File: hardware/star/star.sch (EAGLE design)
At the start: 520 parts, among them IC1 MAX481CSA, IC10 MAX481CSA, IC11 MAX481CSA, IC12 MAX481CSA, IC13 MAX481CSA, IC14 MAX481CSA, IC15 MAX481CSA, IC16 MAX481CSA, IC17 MAX481CSA, IC18 MAX481CSA, IC19 MAX481CSA, IC2 LD117AS12TR, IC20 MAX481CSA, IC21 MAX481CSA, IC22 LD117AS12TR, IC23 LD117AS12TR, IC3 MAX481CSA, IC4 MAX481CSA, IC5 MAX481CSA, IC6 MAX481CSA, IC7 MAX481CSA, IC8 MAX481CSA, IC9 MAX481CSA

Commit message: Progress
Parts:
- removed ACCESSORY, ACCESSORY_GPIO: (no value), pinhead:PINHD-1X5
- removed C100, C101, C102, C103, C104, C105, C106, C107, C108, C109, C110, C111, C112, C113, C114, C115, C116, C117, C118, C119, C120, C121, C122, C123, C124, C37, C38, C39, C40, C41, C42, C43, C44, C45, C46, C47, C48, C49, C50, C51, C52, C53, C54, C55, C56, C57, C58, C59, C60, C61, C62, C63, C64, C65, C66, C67, C68, C73, C74, C75, C76, C77, C78, C79, C80, C81, C82, C83, C84, C85, C86, C87, C88, C93, C94, C95, C96, C97, C98, C99: 1nf, rcl:C-USC0603
- removed C24, C25, C26, C27, C28, C29, C30, C31, C32, C33, C90: 1uf, rcl:C-USC0805
- removed C34, C91, C92: 10uf, rcl:C-USC0603
- removed C69, C70, C71, C72: 2200uf, rcl:CPOL-USE5-13
- removed D10, D11, D12, D13, D14, D15, D16, D17, D18, D19, D20, D21, D22, D23, D24, D25, D26, D27, D28, D29, D30, D31, D32, D33, D34, D35, D36, D37, D38, D39, D40, D41, D42, D43, D44, D45, D46, D47, D48, D49, D50, D51, D52, D53, D54, D55, D56, D57, D58, D59, D60, D61, D62, D63, D64, D65, D66, D67, D68, D69, D70, D71, D72, D73, D74, D75, D76, D77, D78, D79, D80: (no value), SparkFun-LED:LED0603
- removed D81, D86: red, SparkFun-LED:LED0603
- removed D82, D87: green, SparkFun-LED:LED0603
- removed D83, D88: blue, SparkFun-LED:LED0603
- removed D84, D89: white, SparkFun-LED:LED0603
- removed D85, D90: yellow, SparkFun-LED:LED0603
- removed GAME_INTERFACE: B12B-PH-K, con-jst-ph:B12B-PH-K
- removed IC10, IC11, IC12, IC13, IC14, IC15, IC16, IC17, IC18, IC19, IC20, IC21, IC5, IC6, IC7, IC8, IC9: MAX481CSA, maxim:MAX481CSA
- removed IC23: LD117AS12TR, v-reg:LD117AS12TR
- removed J1: (no value), SparkFun-Connectors:CONN_02JST-PTH-2
- removed JP1: (no value), pinhead:PINHD-1X2
- removed JP2: (no value), pinhead:PINHD-1X4
- removed NEBULA_B, NEBULA_C, NEBULA_D, NEBULA_E, NEBULA_F, NEBULA_G, NEBULA_H: MCP23017-E/SO, MCP23017-E_SO:MCP23017-E/SO
- removed R100, R101, R102, R133, R134, R135, R136, R137, R50, R51, R52, R53, R66, R67, R69, R70, R71, R72, R73, R74, R75, R76, R77, R78, R79, R80, R81, R82, R87, R88, R89, R90, R91, R92, R93, R94, R95, R96, R97, R98, R99: 10k, rcl:R-US_R0603
- removed R103, R104, R105, R106, R140, R141, R142, R143, R144, R145, R146, R147, R148, R149, R150, R151, R152, R153, R154, R155, R156, R157, R158, R159, R160, R161, R162, R163, R164, R165, R166, R167, R168, R169, R170, R171, R172, R173, R174, R175, R176, R177, R178, R179, R180, R181, R182, R183, R184, R185, R186, R187, R188, R189, R190, R191, R192, R193, R194, R195, R196, R197, R198, R199, R200, R201, R202, R203, R204, R205, R206, R207, R208, R209, R210, R211, R212, R213, R214, R215, R216, R217, R218, R219, R54, R55, R56, R57, R58, R59, R60, R61, R62, R63, R64, R65, R83, R84, R85, R86: 68, rcl:R-US_R0603
- removed R107, R108, R109, R110, R111, R112, R113, R114, R115, R116, R117, R118, R119, R120, R121, R122, R123, R124: 120, rcl:R-US_R0603
- removed R125, R126, R127, R128, R129: 1k, rcl:R-US_R0603
- removed R138, R68: 10, rcl:R-US_R1206
- removed S1, S2, S3, S4, S5: MOMENTARY-SWITCH-SPST-PTH-6.0MM, SparkFun-Switches:MOMENTARY-SWITCH-SPST-PTH-6.0MM
- removed STAR_10, STAR_11, STAR_12, STAR_13, STAR_14, STAR_15, STAR_16, STAR_17, STAR_18, STAR_19, STAR_2, STAR_20, STAR_3, STAR_4, STAR_5, STAR_6, STAR_7, STAR_8, STAR_9: B8B-PH-K, con-jst-ph:B8B-PH-K
- removed ULN10, ULN11, ULN12, ULN2, ULN3, ULN4, ULN5, ULN6, ULN7, ULN8, ULN9: (no value), SparkFun-IC-Special-Function:ULN2803SOICW
- added K1, K2: T90-12VDC-TL-A, relay:JT1A-PCB-DC12V
- added T1, T2, T3, T4: T_PNP_MMBT5401_CHANGJ_SOT23-BEC, JLC PCB Basic Parts_loc:T_PNP_MMBT5401_CHANGJ_SOT23-BEC
- added U1: TCLT1600, TCLT1600:TCLT1600
- added ULN1: (no value), SparkFun-IC-Special-Function:ULN2803SOICW
- added X1: MKDSN1,5/2-5,08, con-phoenix-508:MKDSN1,5/2-5,08
- added X3: MKDSN1,5/5-5,08, con-phoenix-508:MKDSN1,5/5-5,08
- C10, C11, C12, C9: value 10uf -> C_100UF/6.3V_1206; device rcl:C-USC0603 -> JLC PCB Basic Parts_loc:C_100UF/6.3V_1206; LCSC_PART C19702 -> (none)
- C13: value 10uf -> C_1NF/2KV_1206; device rcl:C-USC0603 -> JLC PCB Basic Parts_loc:C_1NF/2KV_1206; LCSC_PART C19702 -> (none)
- C15, C19, C21, C23: value 1uf -> C_100PF/50V_0603; device rcl:C-USC0805 -> JLC PCB Basic Parts_loc:C_100PF/50V_0603; LCSC_PART C15849 -> (none)
- C16, C17: value 1uf -> C_1NF/50V_0603; device rcl:C-USC0805 -> JLC PCB Basic Parts_loc:C_1NF/50V_0603; LCSC_PART C15849 -> (none)
- C18, C20, C22: value 1uf -> C_1NF/2KV_1206; device rcl:C-USC0805 -> JLC PCB Basic Parts_loc:C_1NF/2KV_1206; LCSC_PART C15849 -> (none)
- C7: value 10uf -> C_1NF/50V_0603; device rcl:C-USC0603 -> JLC PCB Basic Parts_loc:C_1NF/50V_0603; LCSC_PART C19702 -> (none)
- D1: value (none) -> red; JLC_ROTATION (none) -> 180
- D6: value (none) -> green; JLC_ROTATION (none) -> 180; LCSC_PART C2286 -> C72043
- D7: value (none) -> green; JLC_ROTATION (none) -> 180
- D8: value (none) -> green; JLC_ROTATION (none) -> 180; LCSC_PART C72041 -> C72043
- D9: value (none) -> green; JLC_ROTATION (none) -> 180; LCSC_PART C2290 -> C72043
- D91, D92, D93, D94: JLC_ROTATION (none) -> 180
- IC3: value MAX481CSA -> 74HCT08D; device maxim:MAX481CSA -> 74xx-eu:74HCT08D; LCSC_PART C8963 -> C5593
- IC4: value MAX481CSA -> 7404D; device maxim:MAX481CSA -> 74xx-us:7404D; LCSC_PART C8963 -> C5590
- R10, R11, R12, R13: value 10k -> R_4.7K_1206; device rcl:R-US_R0603 -> JLC PCB Basic Parts_loc:R_4.7K_1206; LCSC_PART C25804 -> (none)
- R14, R21, R23, R30, R32, R37, R39, R44: value 10k -> R_2K_0603; device rcl:R-US_R0603 -> JLC PCB Basic Parts_loc:R_2K_0603; LCSC_PART C25804 -> (none)
- R15, R24, R33, R40: value 10k -> R_10R_0603; device rcl:R-US_R0603 -> JLC PCB Basic Parts_loc:R_10R_0603; LCSC_PART C25804 -> (none)
- R16, R25, R34, R41: value 10k -> R_12K_0603; device rcl:R-US_R0603 -> JLC PCB Basic Parts_loc:R_12K_0603; LCSC_PART C25804 -> (none)
- R17, R28, R35, R42: value 10k -> R_2.7K_0603; device rcl:R-US_R0603 -> JLC PCB Basic Parts_loc:R_2.7K_0603; LCSC_PART C25804 -> (none)
- R18, R29, R36, R43: value 10k -> R_1K_0603; device rcl:R-US_R0603 -> JLC PCB Basic Parts_loc:R_1K_0603; LCSC_PART C25804 -> (none)
- R19, R20: value 10k -> R_5.1K_0603; device rcl:R-US_R0603 -> JLC PCB Basic Parts_loc:R_5.1K_0603; LCSC_PART C25804 -> (none)
- R2: value 120 -> R_150R_0603; device rcl:R-US_R0603 -> JLC PCB Basic Parts_loc:R_150R_0603; LCSC_PART C22787 -> (none)
- R22, R31, R38, R9: value 10k -> R_7.5K_0603; device rcl:R-US_R0603 -> JLC PCB Basic Parts_loc:R_7.5K_0603; LCSC_PART C25804 -> (none)
- R45, R46, R47, R48: value 10k -> R_6.2K_0603; device rcl:R-US_R0603 -> JLC PCB Basic Parts_loc:R_6.2K_0603; LCSC_PART C25804 -> (none)
- R49: value 10k -> R_0R_0603; device rcl:R-US_R0603 -> JLC PCB Basic Parts_loc:R_0R_0603; LCSC_PART C25804 -> (none)
- R7, R8: value 10k -> 1k; LCSC_PART C25804 -> C21190
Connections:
- removed net B0: NEBULA_B.GPA0, ULN5.8
- removed net B1: NEBULA_B.GPA1, ULN5.7
- removed net B10: NEBULA_B.GPB2, ULN6.6
- removed net B11: NEBULA_B.GPB3, ULN6.5
- removed net B12: NEBULA_B.GPB4, ULN6.4
- removed net B13: NEBULA_B.GPB5, ULN6.3
- removed net B14: NEBULA_B.GPB6, ULN6.2
- removed net B15: NEBULA_B.GPB7, ULN6.1
- removed net B2: NEBULA_B.GPA2, ULN5.6
- removed net B3: NEBULA_B.GPA3, ULN5.5
- removed net B4: NEBULA_B.GPA4, ULN5.4
- removed net B5: NEBULA_B.GPA5, ULN5.3
- removed net B6: NEBULA_B.GPA6, ULN5.2
- removed net B7: NEBULA_B.GPA7, ULN5.1
- removed net B8: NEBULA_B.GPB0, ULN6.8
- removed net B9: NEBULA_B.GPB1, ULN6.7
- removed net C0: NEBULA_C.GPA0, ULN7.8
- removed net C1: NEBULA_C.GPA1, ULN7.7
- removed net C10: NEBULA_C.GPB2, ULN8.6
- removed net C11: NEBULA_C.GPB3, ULN8.5
- removed net C12: NEBULA_C.GPB4, ULN8.4
- removed net C13: NEBULA_C.GPB5, ULN8.3
- removed net C14: NEBULA_C.GPB6, ULN8.2
- removed net C15: NEBULA_C.GPB7, ULN8.1
- removed net C2: NEBULA_C.GPA2, ULN7.6
- removed net C3: NEBULA_C.GPA3, ULN7.5
- removed net C4: NEBULA_C.GPA4, ULN7.4
- removed net C5: NEBULA_C.GPA5, ULN7.3
- removed net C6: NEBULA_C.GPA6, ULN7.2
- removed net C7: NEBULA_C.GPA7, ULN7.1
- removed net C8: NEBULA_C.GPB0, ULN8.8
- removed net C9: NEBULA_C.GPB1, ULN8.7
- removed net D0: NEBULA_D.GPA0, ULN9.8
- removed net D1: NEBULA_D.GPA1, ULN9.7
- removed net D10: NEBULA_D.GPB2, ULN10.6
- removed net D11: NEBULA_D.GPB3, ULN10.5
- removed net D12: NEBULA_D.GPB4, ULN10.4
- removed net D13: NEBULA_D.GPB5, ULN10.3
- removed net D14: NEBULA_D.GPB6, ULN10.2
- removed net D15: NEBULA_D.GPB7, ULN10.1
- removed net D2: NEBULA_D.GPA2, ULN9.6
- removed net D3: NEBULA_D.GPA3, ULN9.5
- removed net D4: NEBULA_D.GPA4, ULN9.4
- removed net D5: NEBULA_D.GPA5, ULN9.3
- removed net D6: NEBULA_D.GPA6, ULN9.2
- removed net D7: NEBULA_D.GPA7, ULN9.1
- removed net D8: NEBULA_D.GPB0, ULN10.8
- removed net D9: NEBULA_D.GPB1, ULN10.7
- removed net E0: NEBULA_E.GPA0, ULN11.8
- removed net E1: NEBULA_E.GPA1, ULN11.7
- removed net E10: NEBULA_E.GPB2, ULN12.6
- removed net E11: NEBULA_E.GPB3, ULN12.5
- removed net E12: NEBULA_E.GPB4, ULN12.4
- removed net E13: NEBULA_E.GPB5, ULN12.3
- removed net E14: NEBULA_E.GPB6, ULN12.2
- removed net E15: NEBULA_E.GPB7, ULN12.1
- removed net E2: NEBULA_E.GPA2, ULN11.6
- removed net E3: NEBULA_E.GPA3, ULN11.5
- removed net E4: NEBULA_E.GPA4, ULN11.4
- removed net E5: NEBULA_E.GPA5, ULN11.3
- removed net E6: NEBULA_E.GPA6, ULN11.2
- removed net E7: NEBULA_E.GPA7, ULN11.1
- removed net E8: NEBULA_E.GPB0, ULN12.8
- removed net E9: NEBULA_E.GPB1, ULN12.7
- removed net F0: IC1G$1.RE/, NEBULA_F.GPA0
- removed net F1: IC1G$1.DE, NEBULA_F.GPA1
- removed net F10: IC7G$1.RE/, NEBULA_F.GPB2
- removed net F11: IC7G$1.DE, NEBULA_F.GPB3
- removed net F12: IC8G$1.RE/, NEBULA_F.GPB4
- removed net F13: IC8G$1.DE, NEBULA_F.GPB5
- removed net F14: IC9G$1.RE/, NEBULA_F.GPB6
- removed net F15: IC9G$1.DE, NEBULA_F.GPB7
- removed net F2: IC3G$1.RE/, NEBULA_F.GPA2
- removed net F3: IC3G$1.DE, NEBULA_F.GPA3
- removed net F4: IC4G$1.RE/, NEBULA_F.GPA4
- removed net F5: IC4G$1.DE, NEBULA_F.GPA5
- removed net F6: IC5G$1.RE/, NEBULA_F.GPA6
- removed net F7: IC5G$1.DE, NEBULA_F.GPA7
- removed net F8: IC6G$1.RE/, NEBULA_F.GPB0
- removed net F9: IC6G$1.DE, NEBULA_F.GPB1
- removed net G0: IC10G$1.RE/, NEBULA_G.GPA0
- removed net G1: IC10G$1.DE, NEBULA_G.GPA1
- removed net G10: IC15G$1.RE/, NEBULA_G.GPB2
- removed net G11: IC15G$1.DE, NEBULA_G.GPB3
- removed net G12: IC16G$1.RE/, NEBULA_G.GPB4
- removed net G13: IC16G$1.DE, NEBULA_G.GPB5
- removed net G14: IC17G$1.RE/, NEBULA_G.GPB6
- removed net G15: IC17G$1.DE, NEBULA_G.GPB7
- removed net G2: IC11G$1.RE/, NEBULA_G.GPA2
- removed net G3: IC11G$1.DE, NEBULA_G.GPA3
- removed net G4: IC12G$1.RE/, NEBULA_G.GPA4
- removed net G5: IC12G$1.DE, NEBULA_G.GPA5
- removed net G6: IC13G$1.RE/, NEBULA_G.GPA6
- removed net G7: IC13G$1.DE, NEBULA_G.GPA7
- removed net G8: IC14G$1.RE/, NEBULA_G.GPB0
- removed net G9: IC14G$1.DE, NEBULA_G.GPB1
- removed net H0: IC18G$1.RE/, NEBULA_H.GPA0
- removed net H1: IC18G$1.DE, NEBULA_H.GPA1
- removed net H10: D88.C, GAME_INTERFACE.4, NEBULA_H.GPB2, R135.2, S3.1
- removed net H11: D90.C, GAME_INTERFACE.5, NEBULA_H.GPB3, R134.2, S4.1
- removed net H12: D89.C, GAME_INTERFACE.6, NEBULA_H.GPB4, R133.2, S5.1
- removed net H13: ACCESSORY_GPIO.2, NEBULA_H.GPB5, ULN2.3
- removed net H14: ACCESSORY_GPIO.3, NEBULA_H.GPB6, ULN2.2
- removed net H15: ACCESSORY_GPIO.4, NEBULA_H.GPB7, ULN2.1
- removed net H2: IC19G$1.RE/, NEBULA_H.GPA2
- removed net H3: IC19G$1.DE, NEBULA_H.GPA3
- removed net H4: IC20G$1.RE/, NEBULA_H.GPA4
- removed net H5: IC20G$1.DE, NEBULA_H.GPA5
- removed net H6: IC21G$1.RE/, NEBULA_H.GPA6
- removed net H7: IC21G$1.DE, NEBULA_H.GPA7
- removed net H8: D86.C, GAME_INTERFACE.2, NEBULA_H.GPB0, R137.2, S1.1
- removed net H9: D87.C, GAME_INTERFACE.3, NEBULA_H.GPB1, R136.2, S2.1
- removed net N$100: D77.C, R99.2
- removed net N$101: D78.C, R100.2
- removed net N$102: D79.C, R101.2
- removed net N$103: D80.C, R102.2
- removed net N$104: R104.2, STAR_18.6
- removed net N$105: R105.2, STAR_19.6
- removed net N$106: R106.2, STAR_20.6
- removed net N$107: R103.2, STAR_17.6
- removed net N$110: IC3G$1.B, R2.2, STAR_2.7
- removed net N$111: IC3G$1.A, R2.1, STAR_2.8
- removed net N$112: IC4G$1.B, R107.2, STAR_3.7
- removed net N$113: IC4G$1.A, R107.1, STAR_3.8
- removed net N$114: IC5G$1.B, R108.2, STAR_4.7
- removed net N$115: IC5G$1.A, R108.1, STAR_4.8
- removed net N$116: IC6G$1.B, R109.2, STAR_5.7
- removed net N$117: IC6G$1.A, R109.1, STAR_5.8
- removed net N$118: IC7G$1.B, R110.2, STAR_6.7
- removed net N$119: IC7G$1.A, R110.1, STAR_6.8
- removed net N$120: IC8G$1.B, R111.2, STAR_7.7
- removed net N$121: IC8G$1.A, R111.1, STAR_7.8
- removed net N$122: IC9G$1.B, R112.2, STAR_8.7
- removed net N$123: IC9G$1.A, R112.1, STAR_8.8
- removed net N$124: IC10G$1.B, R113.2, STAR_9.7
- removed net N$125: IC10G$1.A, R113.1, STAR_9.8
- removed net N$126: IC11G$1.B, R114.2, STAR_10.7
- removed net N$127: IC11G$1.A, R114.1, STAR_10.8
- removed net N$128: IC12G$1.B, R115.2, STAR_11.7
- removed net N$129: IC12G$1.A, R115.1, STAR_11.8
- removed net N$130: IC13G$1.B, R116.2, STAR_12.7
- removed net N$131: IC13G$1.A, R116.1, STAR_12.8
- removed net N$132: IC14G$1.B, R117.2, STAR_13.7
- removed net N$133: IC14G$1.A, R117.1, STAR_13.8
- removed net N$134: IC15G$1.B, R118.2, STAR_14.7
- removed net N$135: IC15G$1.A, R118.1, STAR_14.8
- removed net N$136: IC16G$1.B, R119.2, STAR_15.7
- removed net N$137: IC16G$1.A, R119.1, STAR_15.8
- removed net N$138: IC17G$1.B, R120.2, STAR_16.7
- removed net N$139: IC17G$1.A, R120.1, STAR_16.8
- removed net N$140: IC18G$1.B, R121.2, STAR_17.7
- removed net N$141: IC18G$1.A, R121.1, STAR_17.8
- removed net N$142: IC19G$1.B, R122.2, STAR_18.7
- removed net N$143: IC19G$1.A, R122.1, STAR_18.8
- removed net N$144: IC20G$1.B, R123.2, STAR_19.7
- removed net N$145: IC20G$1.A, R123.1, STAR_19.8
- removed net N$146: IC21G$1.B, R124.2, STAR_20.7
- removed net N$147: IC21G$1.A, R124.1, STAR_20.8
- removed net N$148: ACCESSORY.2, ULN2.16
- removed net N$149: ACCESSORY.3, ULN2.17
- removed net N$150: ACCESSORY.4, ULN2.18
- removed net N$151: D84.A, R129.2
- removed net N$152: D85.A, R128.2
- removed net N$153: D83.A, R127.2
- removed net N$154: D82.A, R126.2
- removed net N$155: D81.A, R125.2
- removed net N$160: C37.1, R143.1, R3.1, ULN3.11
- removed net N$161: C38.1, R142.1, R4.1, ULN3.12
- removed net N$162: C39.1, R141.1, R5.1, ULN3.13
- removed net N$163: C40.1, R140.1, R6.1, ULN3.14
- removed net N$164: C44.1, R10.1, R144.1, ULN3.18
- removed net N$165: C43.1, R145.1, R9.1, ULN3.17
- removed net N$166: C42.1, R146.1, R8.1, ULN3.16
- removed net N$167: C41.1, R147.1, R7.1, ULN3.15
- removed net N$168: R143.2, STAR_1.2
- removed net N$169: R142.2, STAR_1.3
- removed net N$170: R141.2, STAR_1.4
- removed net N$171: R140.2, STAR_1.5
- removed net N$172: R147.2, STAR_2.2
- removed net N$173: R146.2, STAR_2.3
- removed net N$174: R145.2, STAR_2.4
- removed net N$175: R144.2, STAR_2.5
- removed net N$176: R151.2, STAR_3.2
- removed net N$177: R150.2, STAR_3.3
- removed net N$178: R149.2, STAR_3.4
- removed net N$179: R148.2, STAR_3.5
- removed net N$180: R155.2, STAR_4.2
- removed net N$181: R154.2, STAR_4.3
- removed net N$182: R153.2, STAR_4.4
- removed net N$183: R152.2, STAR_4.5
- removed net N$184: C45.1, R11.1, R151.1, ULN4.11
- removed net N$185: C46.1, R12.1, R150.1, ULN4.12
- removed net N$186: C47.1, R13.1, R149.1, ULN4.13
- removed net N$187: C48.1, R14.1, R148.1, ULN4.14
- removed net N$188: C52.1, R152.1, R18.1, ULN4.18
- removed net N$189: C51.1, R153.1, R17.1, ULN4.17
- removed net N$190: C50.1, R154.1, R16.1, ULN4.16
- removed net N$191: C49.1, R15.1, R155.1, ULN4.15
- removed net N$192: C53.1, R159.1, R19.1, ULN5.11
- removed net N$193: C56.1, R156.1, R22.1, ULN5.14
- removed net N$194: C55.1, R157.1, R21.1, ULN5.13
- removed net N$195: C54.1, R158.1, R20.1, ULN5.12
- removed net N$196: C60.1, R160.1, R28.1, ULN5.18
- removed net N$197: C59.1, R161.1, R25.1, ULN5.17
- removed net N$198: C58.1, R162.1, R24.1, ULN5.16
- removed net N$199: C57.1, R163.1, R23.1, ULN5.15
- removed net N$200: R159.2, STAR_5.2
- removed net N$201: R158.2, STAR_5.3
- removed net N$202: R157.2, STAR_5.4
- removed net N$203: R156.2, STAR_5.5
- removed net N$204: R163.2, STAR_6.2
- removed net N$205: R162.2, STAR_6.3
- removed net N$206: R161.2, STAR_6.4
- removed net N$207: R160.2, STAR_6.5
- removed net N$208: R167.2, STAR_7.2
- removed net N$209: R166.2, STAR_7.3
- removed net N$210: R165.2, STAR_7.4
- removed net N$211: R164.2, STAR_7.5
- removed net N$212: R171.2, STAR_8.2
- removed net N$213: R170.2, STAR_8.3
- removed net N$214: R169.2, STAR_8.4
- removed net N$215: R168.2, STAR_8.5
- removed net N$216: C61.1, R167.1, R29.1, ULN6.11
- removed net N$217: C62.1, R166.1, R30.1, ULN6.12
- removed net N$218: C63.1, R165.1, R31.1, ULN6.13
- removed net N$219: C64.1, R164.1, R32.1, ULN6.14
- removed net N$220: C68.1, R168.1, R36.1, ULN6.18
- removed net N$221: C67.1, R169.1, R35.1, ULN6.17
- removed net N$222: C66.1, R170.1, R34.1, ULN6.16
- removed net N$223: C65.1, R171.1, R33.1, ULN6.15
- removed net N$224: R175.2, STAR_9.2
- removed net N$225: R179.2, STAR_10.2
- removed net N$226: R178.2, STAR_10.3
- removed net N$227: R174.2, STAR_9.3
- removed net N$228: R173.2, STAR_9.4
- removed net N$229: R172.2, STAR_9.5
- removed net N$230: R177.2, STAR_10.4
- removed net N$231: R176.2, STAR_10.5
- removed net N$232: R183.2, STAR_11.2
- removed net N$233: R182.2, STAR_11.3
- removed net N$234: R181.2, STAR_11.4
- removed net N$235: R180.2, STAR_11.5
- removed net N$236: R187.2, STAR_12.2
- removed net N$237: R186.2, STAR_12.3
- removed net N$238: R185.2, STAR_12.4
- removed net N$239: R184.2, STAR_12.5
- removed net N$240: C73.1, R175.1, R37.1, ULN7.11
- removed net N$241: C74.1, R174.1, R38.1, ULN7.12
- removed net N$242: C75.1, R173.1, R39.1, ULN7.13
- removed net N$243: C76.1, R172.1, R40.1, ULN7.14
- removed net N$244: R191.2, STAR_13.2
- removed net N$245: C79.1, R177.1, R43.1, ULN7.17
- removed net N$246: C78.1, R178.1, R42.1, ULN7.16
- removed net N$247: C77.1, R179.1, R41.1, ULN7.15
- removed net N$248: C81.1, R183.1, R45.1, ULN8.11
- removed net N$249: C82.1, R182.1, R46.1, ULN8.12
- removed net N$250: C83.1, R181.1, R47.1, ULN8.13
- removed net N$251: C84.1, R180.1, R48.1, ULN8.14
- removed net N$252: C80.1, R176.1, R44.1, ULN7.18
- removed net N$253: C87.1, R185.1, R51.1, ULN8.17
- removed net N$254: C86.1, R186.1, R50.1, ULN8.16
- removed net N$255: C85.1, R187.1, R49.1, ULN8.15
- removed net N$256: R190.2, STAR_13.3
- removed net N$257: R189.2, STAR_13.4
- removed net N$258: R188.2, STAR_13.5
- removed net N$259: R196.2, STAR_14.2
- removed net N$260: C88.1, R184.1, R52.1, ULN8.18
- removed net N$261: R195.2, STAR_14.3
- removed net N$262: R194.2, STAR_14.4
- removed net N$263: R193.2, STAR_14.5
- removed net N$264: R199.2, STAR_15.2
- removed net N$265: R198.2, STAR_15.3
- removed net N$266: R192.2, STAR_15.5
- removed net N$267: R197.2, STAR_15.4
- removed net N$268: R203.2, STAR_16.2
- removed net N$269: R202.2, STAR_16.3
- removed net N$270: R201.2, STAR_16.4
- removed net N$271: R200.2, STAR_16.5
- removed net N$272: R216.2, STAR_20.5
- removed net N$273: R217.2, STAR_20.4
- removed net N$274: R218.2, STAR_20.3
- removed net N$275: R219.2, STAR_20.2
- removed net N$276: R212.2, STAR_19.5
- removed net N$277: R213.2, STAR_19.4
- removed net N$278: R214.2, STAR_19.3
- removed net N$279: R215.2, STAR_19.2
- removed net N$280: R208.2, STAR_18.5
- removed net N$281: R209.2, STAR_18.4
- removed net N$282: R210.2, STAR_18.3
- removed net N$283: R211.2, STAR_18.2
- removed net N$284: R204.2, STAR_17.5
- removed net N$285: R205.2, STAR_17.4
- removed net N$286: R206.2, STAR_17.3
- removed net N$287: R207.2, STAR_17.2
- removed net N$288: C97.1, R199.1, R75.1, ULN10.11
- removed net N$289: C98.1, R198.1, R76.1, ULN10.12
- removed net N$290: C99.1, R197.1, R77.1, ULN10.13
- removed net N$291: C100.1, R192.1, R78.1, ULN10.14
- removed net N$292: C108.1, R200.1, R82.1, ULN10.18
- removed net N$293: C107.1, R201.1, R81.1, ULN10.17
- removed net N$294: C106.1, R202.1, R80.1, ULN10.16
- removed net N$295: C105.1, R203.1, R79.1, ULN10.15
- removed net N$296: C93.1, R191.1, R53.1, ULN9.11
- removed net N$297: C94.1, R190.1, R66.1, ULN9.12
- removed net N$298: C95.1, R189.1, R69.1, ULN9.13
- removed net N$299: C96.1, R188.1, R70.1, ULN9.14
- removed net N$300: C104.1, R193.1, R74.1, ULN9.18
- removed net N$301: C103.1, R194.1, R73.1, ULN9.17
- removed net N$302: C102.1, R195.1, R72.1, ULN9.16
- removed net N$303: C101.1, R196.1, R71.1, ULN9.15
- removed net N$304: C109.1, R207.1, R87.1, ULN11.11
- removed net N$305: C110.1, R206.1, R88.1, ULN11.12
- removed net N$306: C111.1, R205.1, R89.1, ULN11.13
- removed net N$307: C112.1, R204.1, R90.1, ULN11.14
- removed net N$308: C116.1, R208.1, R94.1, ULN11.18
- removed net N$309: C115.1, R209.1, R93.1, ULN11.17
- removed net N$310: C114.1, R210.1, R92.1, ULN11.16
- removed net N$311: C113.1, R211.1, R91.1, ULN11.15
- removed net N$312: C117.1, R215.1, R95.1, ULN12.11
- removed net N$313: C118.1, R214.1, R96.1, ULN12.12
- removed net N$314: C119.1, R213.1, R97.1, ULN12.13
- removed net N$315: C120.1, R212.1, R98.1, ULN12.14
- removed net N$316: C124.1, R102.1, R216.1, ULN12.18
- removed net N$317: C123.1, R101.1, R217.1, ULN12.17
- removed net N$318: C122.1, R100.1, R218.1, ULN12.16
- removed net N$319: C121.1, R219.1, R99.1, ULN12.15
- removed net N$47: D25.C, R28.2
- removed net N$48: D58.C, R76.2
- removed net N$49: D59.C, R77.2
- removed net N$50: D60.C, R78.2
- removed net N$51: D81.C, GAME_INTERFACE.7, ULN2.11
- removed net N$52: D26.C, R29.2
- removed net N$53: D27.C, R30.2
- removed net N$54: D28.C, R31.2
- removed net N$55: D29.C, R32.2
- removed net N$56: D82.C, GAME_INTERFACE.8, ULN2.12
- removed net N$57: D83.C, GAME_INTERFACE.9, ULN2.13
- removed net N$58: D85.C, GAME_INTERFACE.10, ULN2.14
- removed net N$59: D84.C, GAME_INTERFACE.11, ULN2.15
- removed net N$60: D30.C, R33.2
- removed net N$61: D31.C, R34.2
- removed net N$62: D32.C, R35.2
- removed net N$63: D33.C, R36.2
- removed net N$64: D61.C, R79.2
- removed net N$65: D62.C, R80.2
- removed net N$66: D63.C, R81.2
- removed net N$67: D64.C, R82.2
- removed net N$68: D34.C, R37.2
- removed net N$69: D35.C, R38.2
- removed net N$70: D36.C, R39.2
- removed net N$71: D37.C, R40.2
- removed net N$72: R84.2, STAR_14.6
- removed net N$73: R85.2, STAR_15.6
- removed net N$74: R86.2, STAR_16.6
- removed net N$75: R83.2, STAR_13.6
- removed net N$76: D38.C, R41.2
- removed net N$77: D39.C, R42.2
- removed net N$78: D40.C, R43.2
- removed net N$79: D41.C, R44.2
- removed net N$80: D66.C, R88.2
- removed net N$81: D67.C, R89.2
- removed net N$82: D68.C, R90.2
- removed net N$83: D69.C, R91.2
- removed net N$84: D42.C, R45.2
- removed net N$85: D43.C, R46.2
- removed net N$86: D44.C, R47.2
- removed net N$87: D45.C, R48.2
- removed net N$88: D70.C, R92.2
- removed net N$89: J1.2, JP1.2, R138.1, R68.1
- removed net N$90: D71.C, R93.2
- removed net N$91: D72.C, R94.2
- removed net N$92: D73.C, R95.2
- removed net N$93: D46.C, R49.2
- removed net N$94: D47.C, R50.2
- removed net N$95: D48.C, R51.2
- removed net N$96: D49.C, R52.2
- removed net N$97: D74.C, R96.2
- removed net N$98: D75.C, R97.2
- removed net N$99: D76.C, R98.2
- new net 120_LINE: K1G$2.S, X1-1.KL
- new net 120_NEUTRAL: X1-2.KL, X3-5.KL
- new net BOOMER_BLOWER: C22.1, R38.1, STAR_1.2
- new net BOOMER_FUEL: C20.1, R31.1, STAR_1.3
- new net BOOMER_IGNITER: C18.1, R22.1, STAR_1.4
- new net EN_STATUS: D94.A, IC4C.O
- new net EXP_ULN0: K1G$1.1, ULN1.18
- new net EXP_ULN1: K2G$1.1, ULN1.17
- new net EXP_ULN2: ULN1.16
- new net EXP_ULN3: ULN1.15
- new net EXP_ULN4: ULN1.14
- new net EXP_ULN5: ULN1.13
- new net EXP_ULN6: ULN1.12
- new net EXP_ULN7: ULN1.11
- new net LOCAL_EN: IC4B.O, R21.1, R30.1, R37.1, R44.1, R49.1
- new net POOFER: C13.1, R9.1, STAR_1.5
- new net STAR_ENABLE: R19.1, STAR_1.6
- net +12V: now also K1G$1.2, K2G$1.2, R14.2, R15.2, R23.2, R24.2, R32.2, R33.2, R39.2, R40.2, ULN1.10; no longer ACCESSORY.5, C90.1, C92.1, GAME_INTERFACE.12, IC23.IN, ULN10.10, ULN11.10, ULN12.10, ULN2.10, ULN3.10, ULN4.10, ULN5.10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
- net +3V3: now also R2.2; no longer ACCESSORY_GPIO.5, C10.1, C13.1, C15.1, C16.1, C17.1, C18.1, C19.1, C20.1, C21.1, C22.1, C23.1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
- net +5V: now also C10.1, C9.1; no longer C69.+, C71.+, C91.1, D1.A, D10.A, D11.A, D12.A, D13.A, D14.A, D15.A, D16.A, D17.A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
- net 13: no longer D94.A, J1.1, JP1.1, R103.1, R104.1, R105.1, R106.1, R54.1, R55.1, R56.1, R57.1, R58.1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
- net 16: no longer IC10G$1.RO, IC11G$1.RO, IC12G$1.RO, IC13G$1.RO, IC14G$1.RO, IC15G$1.RO, IC16G$1.RO, IC17G$1.RO, IC18G$1.RO, IC19G$1.RO, IC20G$1.RO, IC21G$1.RO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
- net 17: no longer IC10G$1.DI, IC11G$1.DI, IC12G$1.DI, IC13G$1.DI, IC14G$1.DI, IC15G$1.DI, IC16G$1.DI, IC17G$1.DI, IC18G$1.DI, IC19G$1.DI, IC20G$1.DI, IC21G$1.DI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
- net 18: no longer NEBULA_E.INTB
- net 19: no longer NEBULA_F.INTB
- net 2: no longer JP2.2
- net 21/SDA: no longer NEBULA_B.SDA, NEBULA_C.SDA, NEBULA_D.SDA, NEBULA_E.SDA, NEBULA_F.SDA, NEBULA_G.SDA, NEBULA_H.SDA
- net 22/SCL: no longer NEBULA_B.SCK, NEBULA_C.SCK, NEBULA_D.SCK, NEBULA_E.SCK, NEBULA_F.SCK, NEBULA_G.SCK, NEBULA_H.SCK
- net 23: no longer ULN2.8
- net 25: now also R45.2; no longer ULN2.7
- net 26: now also R46.2; no longer ULN2.6
- net 27: now also R47.2; no longer ULN2.5
- net 32: now also R48.2; no longer ULN2.4
- net 33: no longer NEBULA_G.INTB, NEBULA_H.INTB
- net 35: now also R49.2; no longer NEBULA_B.INTB
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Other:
- note added: "Boomer Blower"
- note added: "Boomer Fuel"
- note added: "Boomer Igniter"
- note added: "Expansion"
- note added: "Expansion x Darlington Array"
- note added: "Fog Machine Interface"
- note added: "Holes"
- note added: "Input Connector & Input RS485"
- note added: "Poofer"
- note added: "Power Input"
- note added: "System Status"
- note added: "Voltage Regulators"
- note removed: "TODO: Power light Safety Engaged Light"
- note removed: "i2c 0x21"
- note removed: "i2c 0x22"
- note removed: "i2c 0x23"
- note removed: "i2c 0x24"
- note removed: "i2c 0x25"
- note removed: "i2c 0x26"
- note removed: "i2c 0x27"
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
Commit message: more progress
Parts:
- removed D2, D3, D4, D5: (no value), SparkFun-LED:LED0603
- removed I2C_1: (no value), pinhead:PINHD-1X4
- removed LEDARRAY: (no value), SparkFun-Connectors:CONN_03LONGPADS
- removed R3, R4, R5, R6: 10k, rcl:R-US_R0603
- removed STAR_1: B8B-PH-K, con-jst-ph:B8B-PH-K
- added 5V_CTRL_LAZERS, STAR_INPUT: B8B-PH-K, con-jst-ph:B8B-PH-K
- added C24, C26, C30: 1uf, rcl:C-USC0805
- added C25, C27, C31: 10uf, rcl:C-USC0603
- added C28: 2200uf, rcl:CPOL-USE5-13
- added C29: (no value), rcl:CPOL-USE10-25
- added C32: C_1UF/50V_0603, JLC PCB Basic Parts_loc:C_1UF/50V_0603
- added D10, D11: MBR20200CT, MBR20200CT:MBR20200CT
- added D12, D13, D14, D15: D_SS210_MDD_SMA, JLC PCB Basic Parts_loc:D_SS210_MDD_SMA
- added D16, D17, D18, D19: blue, SparkFun-LED:LED0603
- added FIRE: MKDSN1,5/8-5,08, con-phoenix-508:MKDSN1,5/8-5,08
- added IC5, IC6, IC7: LM317MABDT, v-reg:LM317MABDT
- added JP1: (no value), pinhead:PINHD-2X2
- added LED_ARRAY: (no value), pinhead:PINHD-1X4
- added Q1, Q2, Q3, Q4: 35A/25V/8.5mΩ, SparkFun-DiscreteSemi:MOSFET-NCH-FDD8780
- added R50, R53, R58: R_240R_0603, JLC PCB Basic Parts_loc:R_240R_0603
- added R51, R54, R59: R_750R_0603, JLC PCB Basic Parts_loc:R_750R_0603
- added R52: R_0R_1206, JLC PCB Basic Parts_loc:R_0R_1206
- added R55, R56, R57: S14K420, varistor:S14K420
- added R60, R61, R62: R_56K_0805, JLC PCB Basic Parts_loc:R_56K_0805
- added R63: R_2.2K_0603, JLC PCB Basic Parts_loc:R_2.2K_0603
- R26, R27: value 10k -> R_3K_0603; device rcl:R-US_R0603 -> JLC PCB Basic Parts_loc:R_3K_0603; LCSC_PART C25804 -> (none)
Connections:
- removed net 25: R45.2, U$1.IO25
- removed net 26: R46.2, U$1.IO26
- removed net 27: R47.2, U$1.IO27
- removed net 32: R48.2, U$1.IO32
- removed net N$3: D2.C, R3.2
- removed net N$4: D3.C, R4.2
- removed net N$5: D4.C, R5.2
- removed net N$6: D5.C, R6.2
- new net +6V: D15.C, D16.A, FIRE-1.KL, IC5.OUT, IC6.OUT, IC7.OUT, R50.2, R53.2, R58.2
- new net 25_POOFER: Q1.G, R45.2, U$1.IO25
- new net 26_BOOM_IGNITER: Q4.G, R46.2, U$1.IO26
- new net 27_BOOM_FUEL: Q2.G, R47.2, U$1.IO27
- new net 32_BOOM_BLOWER: Q3.G, R48.2, U$1.IO32
- new net 60VDC: C29.+, D10.C, D12.C, D13.C, D14.C, D17.A, D18.A, D19.A, FIRE-3.KL, FIRE-5.KL, FIRE-7.KL
- new net GND2: C29.-, D11.A1, D11.A2, Q1.S, Q2.S, Q3.S
- new net GND3: C24.2, C25.2, C26.2, C27.2, C30.2, C31.2, Q4.S, R51.1, R52.2, R54.1, R59.1
- new net N$47: D13.A, FIRE-6.KL, Q2.D, R61.2
- new net N$48: IC6.ADJ, R53.1, R54.2
- new net N$49: D12.A, FIRE-8.KL, Q1.D, R60.2
- new net N$50: IC5.ADJ, R50.1, R51.2
- new net N$51: D14.A, FIRE-4.KL, Q3.D, R62.2
- new net N$52: D15.A, FIRE-2.KL, Q4.D, R63.2
- new net N$53: IC7.ADJ, R58.1, R59.2
- new net N$54: D16.C, R63.1
- new net N$55: D17.C, R62.1
- new net N$56: D18.C, R61.1
- new net N$57: D19.C, R60.1
- net +12V: now also C24.1, C25.1, C26.1, C27.1, C28.+, C30.1, C31.1, IC5.IN, IC6.IN, IC7.IN
- net +3V3: no longer I2C_1.1
- net +5V: now also 5V_CTRL_LAZERS.2, 5V_CTRL_LAZERS.4, 5V_CTRL_LAZERS.6, 5V_CTRL_LAZERS.8, C32.1, LED_ARRAY.1; no longer D2.A, D3.A, D4.A, D5.A, LEDARRAY.3
- net 120_LINE: now also D10.A1, D10.A2, R55.1, R56.1, R57.1
- net 120_NEUTRAL: now also D11.C, R55.2, R56.2, R57.2
- net 18: now also LED_ARRAY.2
- net 19: now also LED_ARRAY.3
- net 21/SDA: now also R27.1; no longer I2C_1.4, R26.1
- net 22/SCL: now also R26.1; no longer I2C_1.3, R27.1
- net 23: now also ULN1.7
- net 33: now also ULN1.8
- net 4: no longer LEDARRAY.2
- net 5: now also ULN1.6
- net A1: now also ULN1.1
- net A10: no longer ULN1.3
- net A11: no longer ULN1.4
- net A12: no longer ULN1.5
- net A13: no longer ULN1.6
- net A14: no longer ULN1.7
- net A15: no longer ULN1.8
- net A2: now also ULN1.2
- net A3: now also ULN1.3
- net A8: no longer ULN1.1
- net A9: no longer ULN1.2
- net BOOMER_BLOWER: now also STAR_INPUT.2; no longer STAR_1.2
- net BOOMER_FUEL: now also STAR_INPUT.3; no longer STAR_1.3
- net BOOMER_IGNITER: now also STAR_INPUT.4; no longer STAR_1.4
- net EXP_ULN2: now also 5V_CTRL_LAZERS.7
- net EXP_ULN5: now also 5V_CTRL_LAZERS.5
- net EXP_ULN6: now also 5V_CTRL_LAZERS.3
- net EXP_ULN7: now also 5V_CTRL_LAZERS.1
- net GND: now also C28.-, C32.2, JP1.1, JP1.2, JP1.3, JP1.4, LED_ARRAY.4, R52.1, STAR_INPUT.1; no longer I2C_1.2, LEDARRAY.1, STAR_1.1
- net N$108: now also STAR_INPUT.7; no longer STAR_1.7
- net N$109: now also STAR_INPUT.8; no longer STAR_1.8
- net POOFER: now also STAR_INPUT.5; no longer STAR_1.5
- net STAR_ENABLE: now also STAR_INPUT.6; no longer STAR_1.6
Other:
- note added: "5v Controlled Output (aka Lasers)"
- note added: "APA 102 LED"
- note added: "Note: ULN7,6,5,2 go to the laser outputs. #2 is on/off only. No PWM possible."
- moved on the sheet: C1, C10, C11, C12, C13, C14, C15, C16, C17, C18, C19, C2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

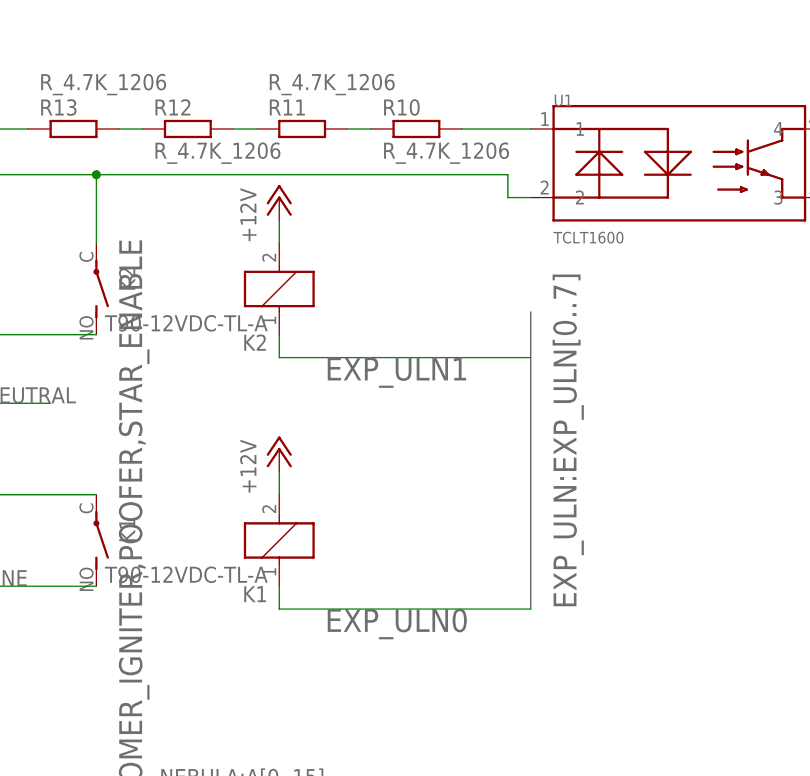
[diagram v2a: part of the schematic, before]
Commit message: progress
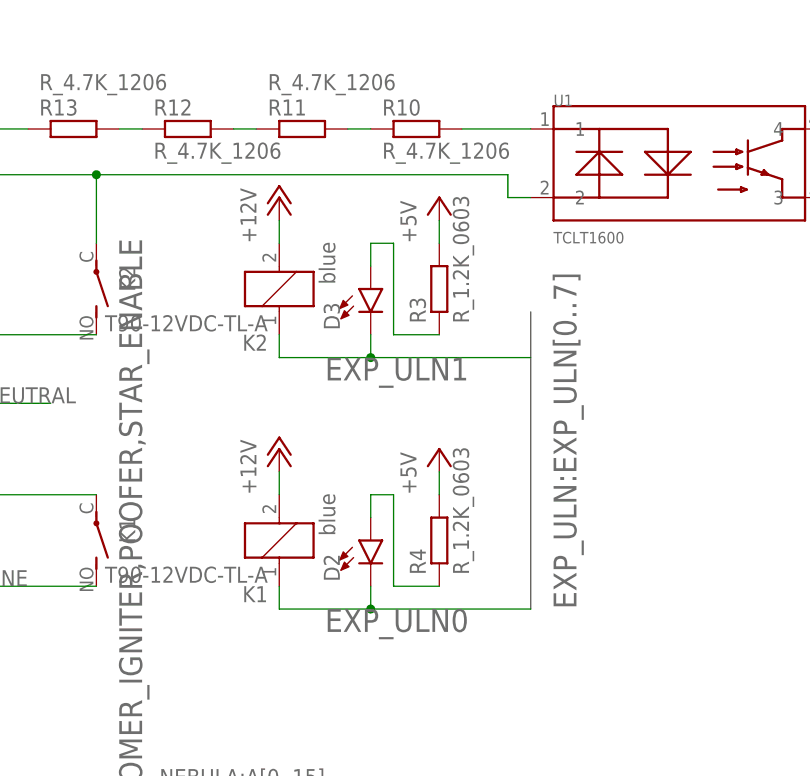
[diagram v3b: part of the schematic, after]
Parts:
- added D2, D3: blue, SparkFun-LED:LED0603
- added R3, R4: R_1.2K_0603, JLC PCB Basic Parts_loc:R_1.2K_0603
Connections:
- new net N$3: D2.A, R4.1
- new net N$4: D3.A, R3.1
- net +5V: now also R3.2, R4.2
- net EXP_ULN0: now also D2.C
- net EXP_ULN1: now also D3.C
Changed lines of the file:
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@@
 <setting verticaltext="up"/>
 </settings>
-<grid distance="0.1" unitdist="inch" unit="inch" style="lines" multiple="1" display="yes" altdistance="0.01" altunitdist="inch" altunit="inch"/>
+<grid distance="0.1" unitdist="inch" unit="inch" style="lines" multiple="1" display="no" altdistance="0.01" altunitdist="inch" altunit="inch"/>
 <layers>
 <layer number="1" name="Top" color="4" fill="1" visible="no" active="no"/>
@@
 <clearance class="5" value="0.254"/>
 </class>
-<class number="6" name="120VAC_PWR" width="2.54" drill="0">
-<clearance class="6" value="1.27"/>
+<class number="6" name="120VAC_PWR" width="1.27" drill="0">
+<clearance class="6" value="0.508"/>
 </class>
 <class number="7" name="120VAC" width="1.27" drill="0">
-<clearance class="7" value="1.27"/>
+<clearance class="7" value="0.508"/>
+</class>
+<class number="8" name="60V" width="1.27" drill="0">
+<clearance class="8" value="0.508"/>
 </class>
 </classes>
@@
 <part name="5V_CTRL_LAZERS" library="con-jst-ph" library_urn="urn:adsk.eagle:library:37597460" deviceset="B8B-PH-K" device="" package3d_urn="urn:adsk.eagle:package:37597503/1"/>
 <part name="P+4" library="supply1" library_urn="urn:adsk.eagle:library:371" deviceset="+5V" device=""/>
+<part name="D2" library="SparkFun-LED" library_urn="urn:adsk.eagle:library:529" deviceset="LED" device="0603" package3d_urn="urn:adsk.eagle:package:39354/1" value="blue">
+<attribute name="JLC_ROTATION" value="180"/>
+<attribute name="LCSC_PART" value="C72041"/>
+</part>
+<part name="D3" library="SparkFun-LED" library_urn="urn:adsk.eagle:library:529" deviceset="LED" device="0603" package3d_urn="urn:adsk.eagle:package:39354/1" value="blue">
+<attribute name="JLC_ROTATION" value="180"/>
+<attribute name="LCSC_PART" value="C72041"/>
+</part>
+<part name="R3" library="JLC PCB Basic Parts_loc" library_urn="urn:adsk.eagle:library:38668506" deviceset="R_" device="_0603" package3d_urn="urn:adsk.eagle:package:23555/3" technology="1.2K"/>
+<part name="R4" library="JLC PCB Basic Parts_loc" library_urn="urn:adsk.eagle:library:38668506" deviceset="R_" device="_0603" package3d_urn="urn:adsk.eagle:package:23555/3" technology="1.2K"/>
+<part name="P+15" library="supply1" library_urn="urn:adsk.eagle:library:371" deviceset="+5V" device=""/>
+<part name="P+25" library="supply1" library_urn="urn:adsk.eagle:library:371" deviceset="+5V" device=""/>
 </parts>
 <sheets>
@@
 <attribute name="VALUE" x="426.72" y="261.62" size="1.778" layer="96" rot="R90"/>
 </instance>
+<instance part="D2" gate="G$1" x="73.66" y="398.78" smashed="yes">
+<attribute name="NAME" x="70.231" y="394.208" size="1.778" layer="95" font="vector" rot="R90"/>
+<attribute name="VALUE" x="67.945" y="399.288" size="1.778" layer="96" font="vector" rot="R90" align="top-left"/>
+<attribute name="LCSC_PART" x="73.66" y="398.78" size="1.778" layer="96" display="off"/>
+<attribute name="JLC_ROTATION" x="73.66" y="398.78" size="1.778" layer="96" display="off"/>
+</instance>
+<instance part="D3" gate="G$1" x="73.66" y="426.72" smashed="yes">
+<attribute name="NAME" x="70.231" y="422.148" size="1.778" layer="95" font="vector" rot="R90"/>
+<attribute name="VALUE" x="67.945" y="427.228" size="1.778" layer="96" font="vector" rot="R90" align="top-left"/>
+<attribute name="LCSC_PART" x="73.66" y="426.72" size="1.778" layer="96" display="off"/>
+<attribute name="JLC_ROTATION" x="73.66" y="426.72" size="1.778" layer="96" display="off"/>
+</instance>
+<instance part="R3" gate="R1" x="81.28" y="426.72" smashed="yes" rot="R90">
+<attribute name="NAME" x="79.7814" y="422.91" size="1.778" layer="95" rot="R90"/>
+<attribute name="VALUE" x="84.582" y="422.91" size="1.778" layer="96" rot="R90"/>
+</instance>
+<instance part="R4" gate="R1" x="81.28" y="398.78" smashed="yes" rot="R90">
+<attribute name="NAME" x="79.7814" y="394.97" size="1.778" layer="95" rot="R90"/>
+<attribute name="VALUE" x="84.582" y="394.97" size="1.778" layer="96" rot="R90"/>
+</instance>
+<instance part="P+15" gate="1" x="81.28" y="436.88" smashed="yes">
+<attribute name="VALUE" x="78.74" y="431.8" size="1.778" layer="96" rot="R90"/>
+</instance>
+<instance part="P+25" gate="1" x="81.28" y="408.94" smashed="yes">
+<attribute name="VALUE" x="78.74" y="403.86" size="1.778" layer="96" rot="R90"/>
+</instance>
 </instances>
 <busses>
@@
 <junction x="429.26" y="259.08"/>
 </segment>
+<segment>
+<pinref part="R4" gate="R1" pin="2"/>
+<pinref part="P+25" gate="1" pin="+5V"/>
+<wire x1="81.28" y1="403.86" x2="81.28" y2="406.4" width="0.1524" layer="91"/>
+</segment>
+<segment>
+<pinref part="R3" gate="R1" pin="2"/>
+<pinref part="P+15" gate="1" pin="+5V"/>
+<wire x1="81.28" y1="431.8" x2="81.28" y2="434.34" width="0.1524" layer="91"/>
+</segment>
 </net>
 <net name="+3V3" class="4">
@@
 <segment>
 <pinref part="K1" gate="G$1" pin="1"/>
-<wire x1="91.44" y1="391.16" x2="63.5" y2="391.16" width="0.1524" layer="91"/>
+<wire x1="91.44" y1="391.16" x2="73.66" y2="391.16" width="0.1524" layer="91"/>
+<wire x1="73.66" y1="391.16" x2="63.5" y2="391.16" width="0.1524" layer="91"/>
 <wire x1="63.5" y1="391.16" x2="63.5" y2="393.7" width="0.1524" layer="91"/>
 <label x="68.58" y="388.62" size="2.54" layer="95"/>
+<pinref part="D2" gate="G$1" pin="C"/>
+<wire x1="73.66" y1="393.7" x2="73.66" y2="391.16" width="0.1524" layer="91"/>
+<junction x="73.66" y="391.16"/>
 </segment>
 </net>
@@
 <segment>
 <pinref part="K2" gate="G$1" pin="1"/>
-<wire x1="91.44" y1="419.1" x2="63.5" y2="419.1" width="0.1524" layer="91"/>
+<wire x1="91.44" y1="419.1" x2="73.66" y2="419.1" width="0.1524" layer="91"/>
+<wire x1="73.66" y1="419.1" x2="63.5" y2="419.1" width="0.1524" layer="91"/>
 <wire x1="63.5" y1="419.1" x2="63.5" y2="421.64" width="0.1524" layer="91"/>
 <label x="68.58" y="416.56" size="2.54" layer="95"/>
+<pinref part="D3" gate="G$1" pin="C"/>
+<wire x1="73.66" y1="421.64" x2="73.66" y2="419.1" width="0.1524" layer="91"/>
+<junction x="73.66" y="419.1"/>
 </segment>
 </net>
@@
 </segment>
 </net>
-<net name="60VDC" class="0">
+<net name="60VDC" class="8">
 <segment>
 <pinref part="D10" gate="G$1" pin="C"/>
@@
 </segment>
 </net>
-<net name="GND2" class="0">
+<net name="GND2" class="8">
 <segment>
 <pinref part="D11" gate="G$1" pin="A1"/>
@@
 </segment>
 </net>
+<net name="N$3" class="0">
+<segment>
+<pinref part="D2" gate="G$1" pin="A"/>
+<wire x1="73.66" y1="401.32" x2="73.66" y2="403.86" width="0.1524" layer="91"/>
+<wire x1="73.66" y1="403.86" x2="76.2" y2="403.86" width="0.1524" layer="91"/>
+<pinref part="R4" gate="R1" pin="1"/>
+<wire x1="76.2" y1="403.86" x2="76.2" y2="393.7" width="0.1524" layer="91"/>
+<wire x1="76.2" y1="393.7" x2="81.28" y2="393.7" width="0.1524" layer="91"/>
+</segment>
+</net>
+<net name="N$4" class="0">
+<segment>
+<pinref part="D3" gate="G$1" pin="A"/>
+<wire x1="73.66" y1="429.26" x2="73.66" y2="431.8" width="0.1524" layer="91"/>
+<wire x1="73.66" y1="431.8" x2="76.2" y2="431.8" width="0.1524" layer="91"/>
+<wire x1="76.2" y1="431.8" x2="76.2" y2="421.64" width="0.1524" layer="91"/>
+<pinref part="R3" gate="R1" pin="1"/>
+<wire x1="76.2" y1="421.64" x2="81.28" y2="421.64" width="0.1524" layer="91"/>
+</segment>
+</net>
